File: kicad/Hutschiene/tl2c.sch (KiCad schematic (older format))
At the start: 32 parts, among them IC101 ATTINY20-X, P101 12VDC, P102 RJ45, P104 TPI Header, P106 240VAC, P108 UG, P109 5VDC, P110 EG, P111 OG, SW101 TL3315NF160Q

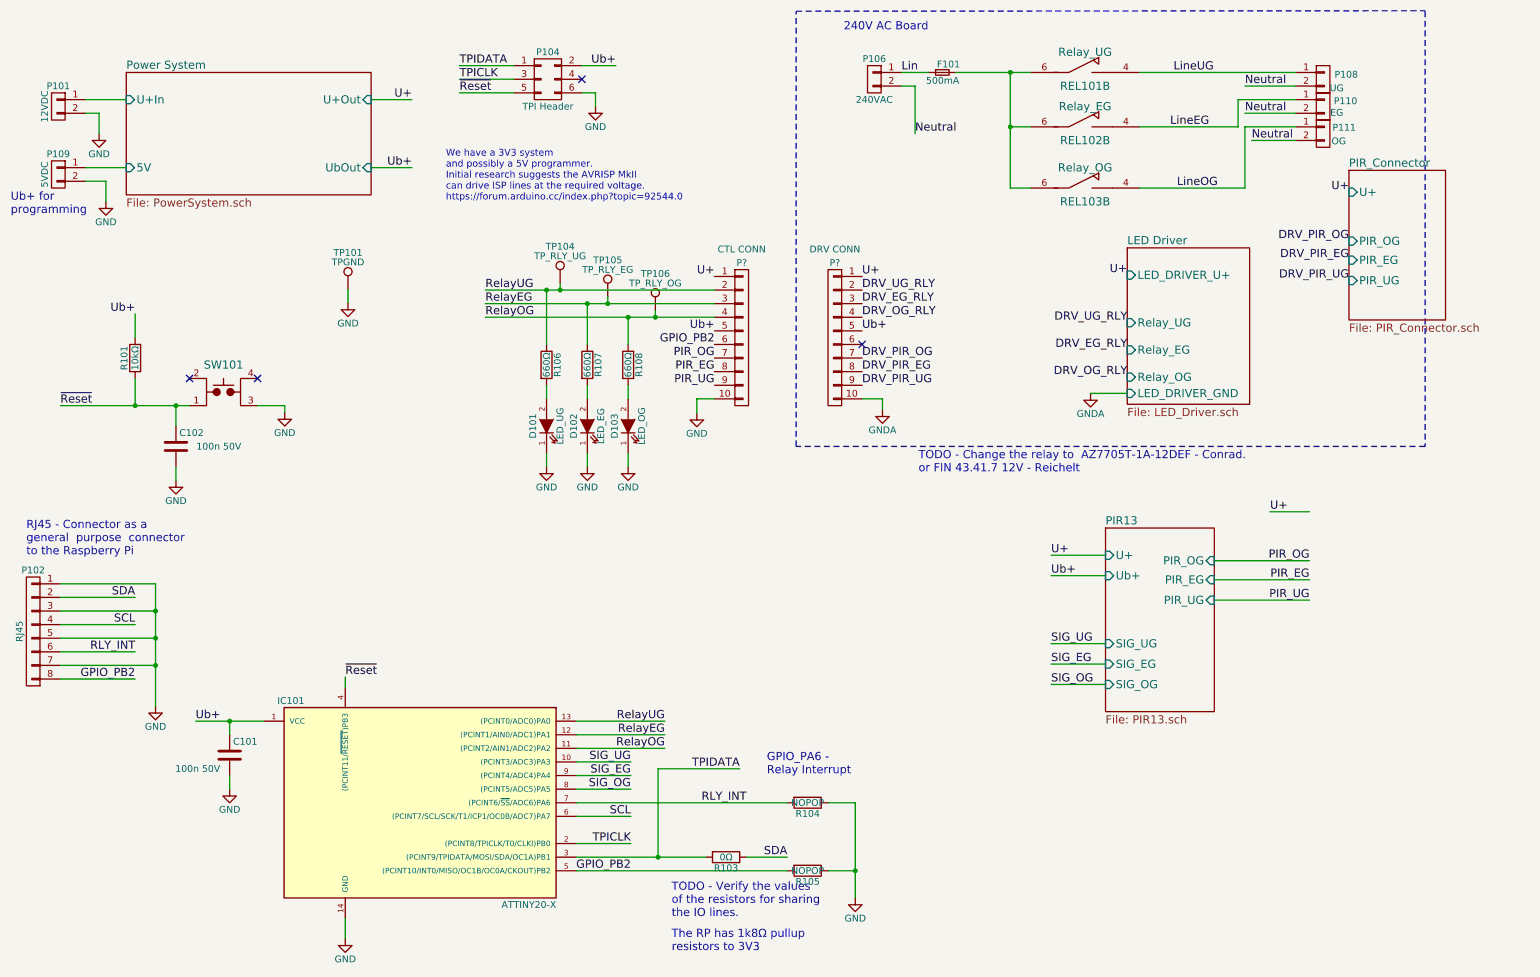
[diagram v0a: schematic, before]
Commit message: Further work on the redesign
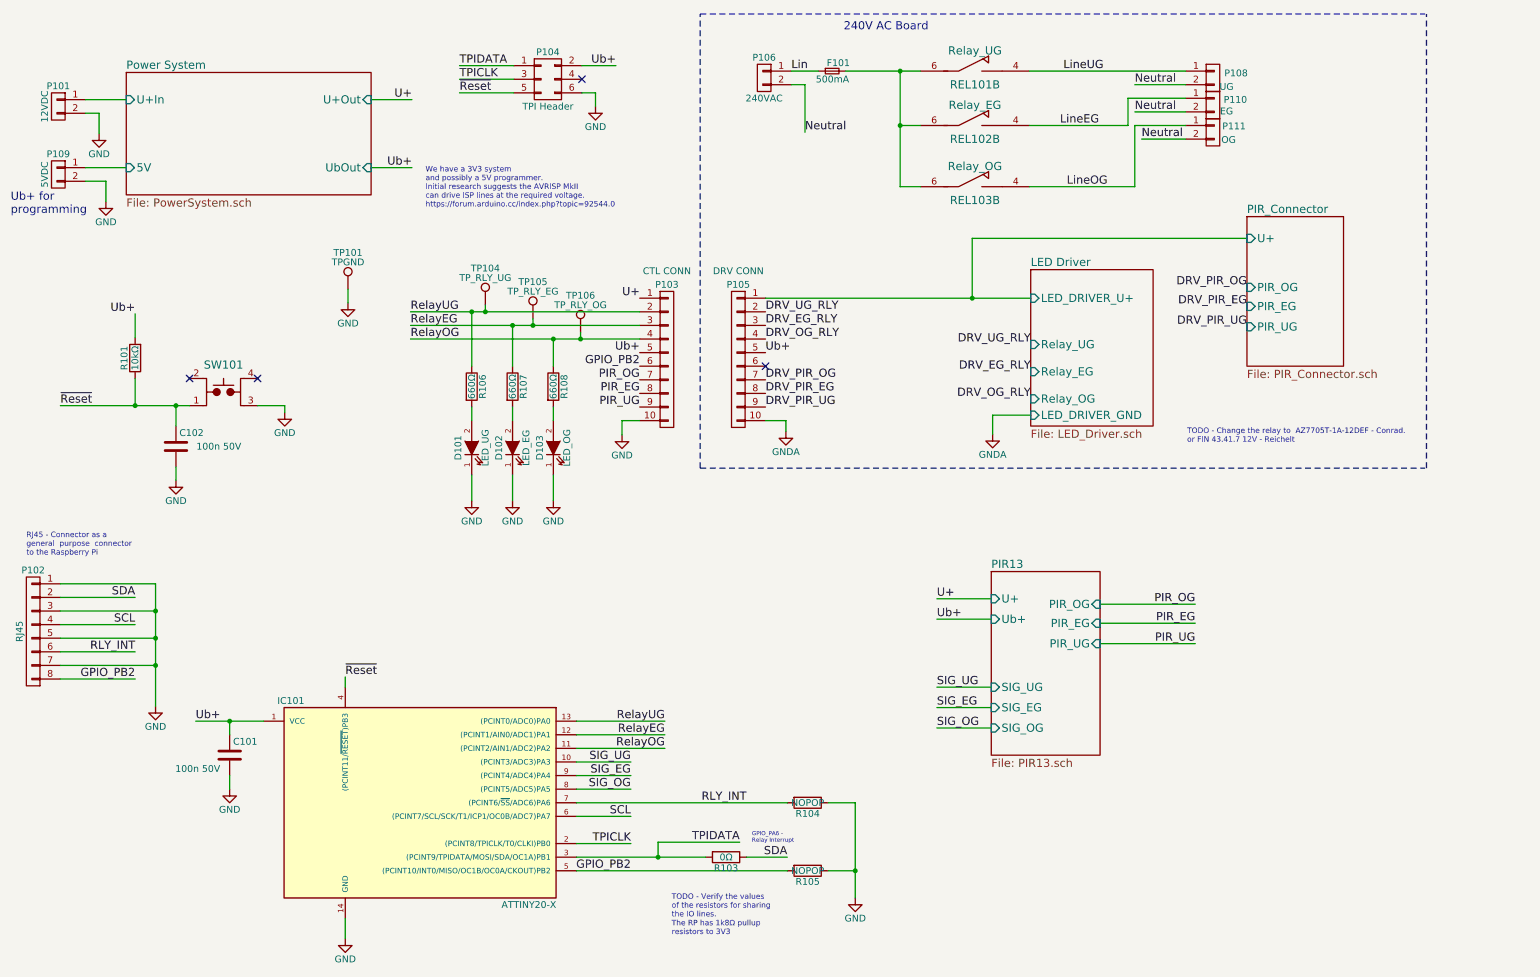
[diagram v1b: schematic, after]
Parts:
- P101: footprint Pin_Headers:Pin_Header_Straight_1x02 -> tl2c-footprint:PCB_Screw_Terminal_Block_5mm_x_2
- P103, P105: renamed from P?; footprint (none) -> Pin_Headers:Pin_Header_Straight_2x05_Pitch2.54mm
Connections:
- net U+: no longer P105.1 (P1)
- new net LED Driver/LED_DRIVER_U+: P105.1 (P1)
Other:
- moved on the sheet: D101, D102, D103, F101, P103, P105, P106, P108, P110, P111, R106, R107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
